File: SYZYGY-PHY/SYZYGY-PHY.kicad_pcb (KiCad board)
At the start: 4 copper layers, 57.7 x 27 mm, 49 parts, among them J1 QTH-020-01-X-D-DP-A, J2 ARJM11C7-502-KB-EW2, J3 Conn_01x11, J4 Conn_01x02, U1 GPY111, U2 TXB0106RGY, U3 TXB0106RGY, Y1 Crystal_GND24

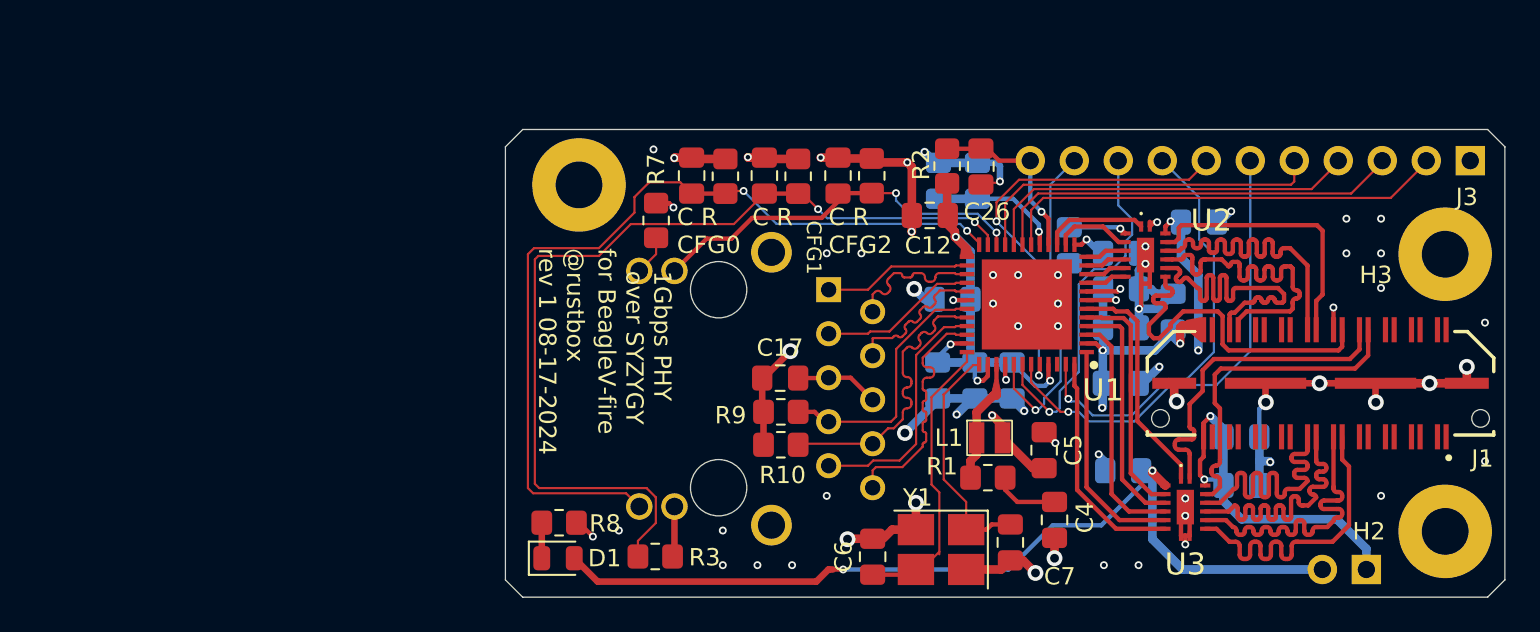
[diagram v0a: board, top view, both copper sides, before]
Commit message: syzygy phy docs
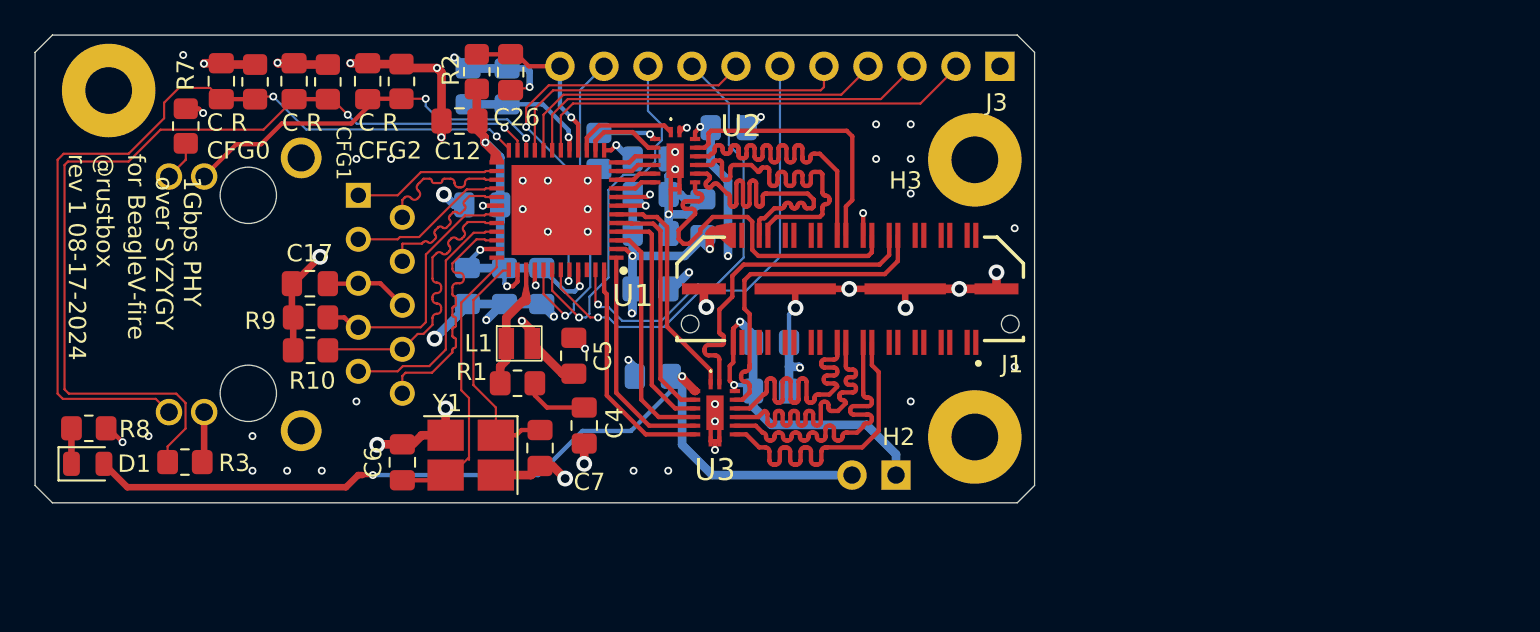
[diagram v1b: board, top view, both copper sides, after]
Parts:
- moved C1 27.7 mm to (105.3, 74.3)
- moved C12 27.7 mm to (87.3, 61.5)
- moved C13 27.7 mm to (88.7, 66.3)
- moved C14 27.7 mm to (87.8, 71.0)
- moved C16 27.7 mm to (87.8, 59.5)
- moved C18 27.7 mm to (90.1, 59.5)
- moved C2 27.7 mm to (101.4, 67.1)
- moved C25 27.7 mm to (105.3, 77.1)
- moved C26 27.7 mm to (90.3, 58.7)
- moved C7 27.7 mm to (92.0, 80.4)
- moved C8 27.7 mm to (92.1, 71.0)
- moved C9 27.7 mm to (98.4, 71.2)
- moved H1 27.7 mm to (67.1, 59.8)
- moved H2 27.7 mm to (117.1, 79.8)
- moved H3 27.7 mm to (117.1, 63.8)
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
